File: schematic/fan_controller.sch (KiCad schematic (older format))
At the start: 10 parts, among them J1 SH1106_OLED, J2 470531000, J3 B3B-EH-A(LF)(SN), SW1 SW_Push, U1 ATmega328P-PU, Y1 16MHz

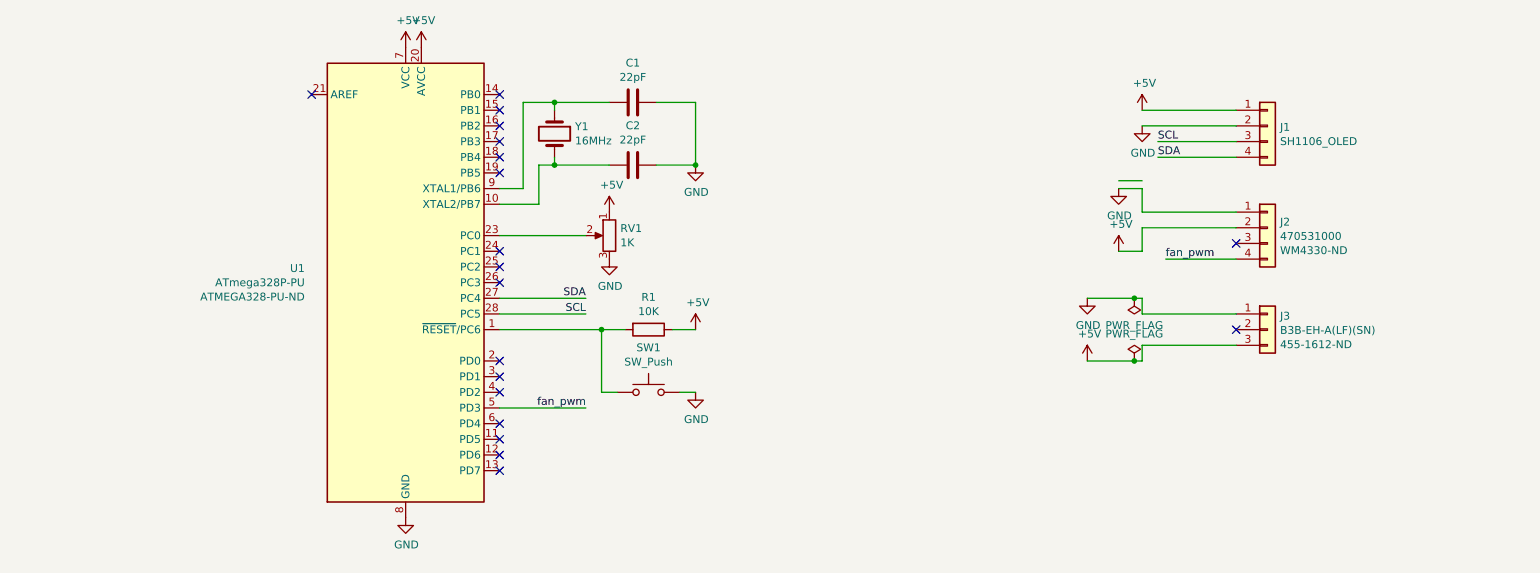
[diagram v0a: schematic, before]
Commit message: Updated schematic
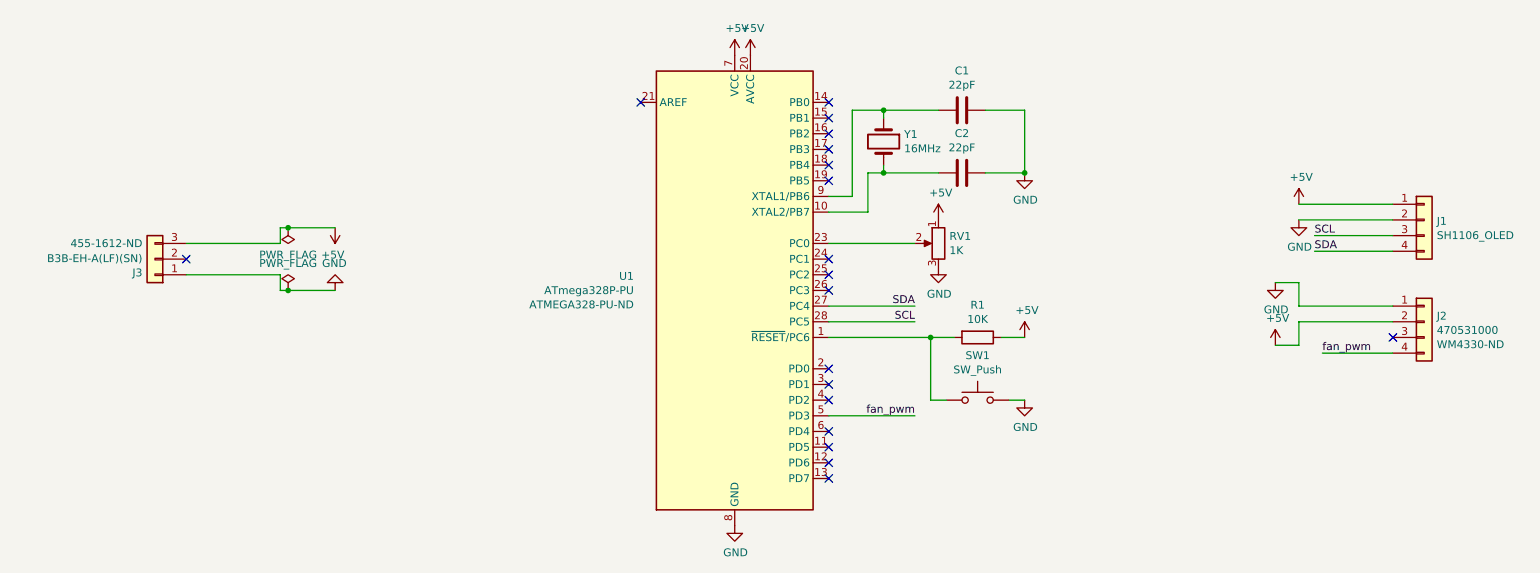
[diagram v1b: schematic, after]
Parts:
- J3: digikey (none) -> 455-1612-ND; digkey 455-1612-ND -> (none)
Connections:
- wire segments 43 -> 42
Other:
- moved on the sheet: C1, C2, J1, J2, J3, R1, RV1, SW1, U1, Y1
